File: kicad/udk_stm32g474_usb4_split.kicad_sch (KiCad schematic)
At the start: 144 parts, among them J1 USB_A, J10 QWIIC, J11 ARGB, J12 5V, J13 USB_C_Receptacle, J14 Conn_01x08_Pin, J15 Conn_01x08_Pin, J16 TC2030-SWD, J17 Conn_01x02_Socket, J18 Conn_01x02_Socket, J2 USB_A, J5 USB_A, J8 SPI, J9 CONN, Q1 AO3401A, SW1 BOOT, SW2 RESET, U1 TS3USB30ERSWR, U10 REF3033E, U11 CH217K, U12 M25C-MEM-SPI, U13 TS3USB30ERSWR, U14 TS3USB30ERSWR, U15 TS3USB30ERSWR, U16 TS3USB30ERSWR, U17 LM66100DCK, U18 LM66100DCK, U19 LM66100DCK, U2 MCP23008-xML, U20 LP5907MFX-3.3, U21 NC7SZ125M5X, U22 LM66100DCK, U3 CH334F, U4 LM66100DCK, U5 LM66100DCK, U6 STM32G474CBTx, U7 TS3USB30ERSWR, U8 LM66100DCK, U9 LM66100DCK, X1 Qwicc Logo, X2 Tecsmith Logo, X3 UDK Logo, X4 OSHW Logo, Y1 12MHz SMD3225-4P, Y2 8MHz SMD3225-4P

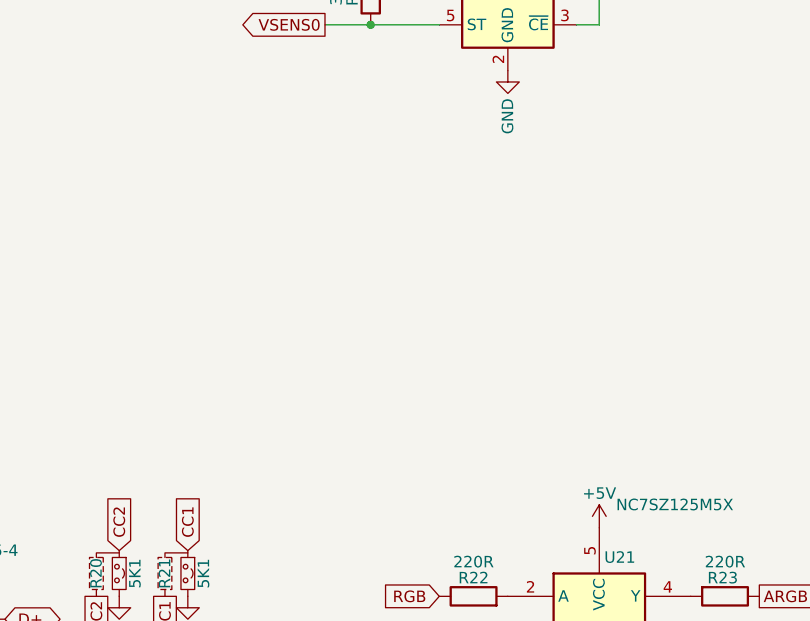
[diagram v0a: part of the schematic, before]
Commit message: added `24AA02E48`
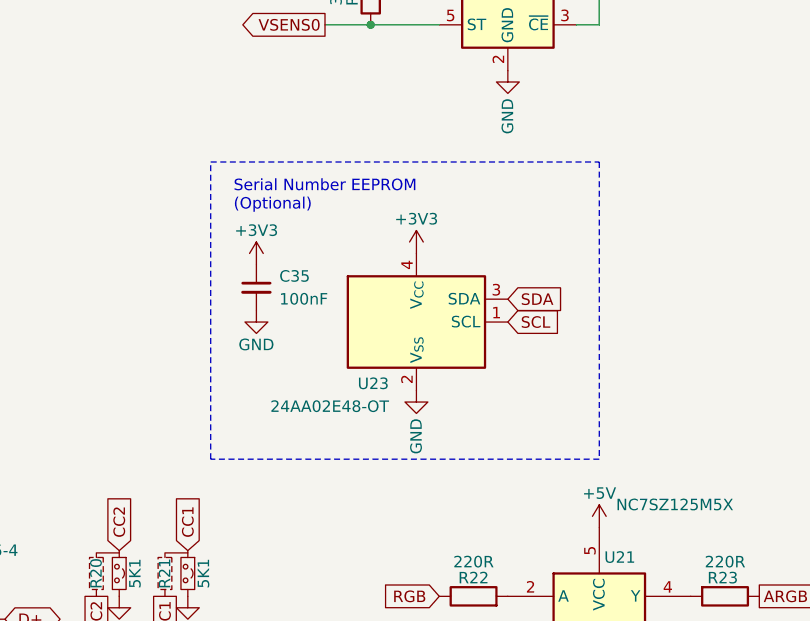
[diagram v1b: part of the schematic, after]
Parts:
- added C35: 100nF, Capacitor_SMD:C_0402_1005Metric, symbol ts-kicad-lib:C
- added U23: 24AA02E48-OT, Package_TO_SOT_SMD:SOT-23-5, symbol Memory_EEPROM:24AA02E-OT
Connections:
- net +3V3: now also C35.1, U23.4 (V_{CC})
- net GND: now also C35.2, U23.2 (V_{SS})
- net I2C1_SCL: now also U23.1 (SCL)
- net I2C1_SDA: now also U23.3 (SDA)
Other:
- note added: "Serial Number EEPROM (Optional)"
